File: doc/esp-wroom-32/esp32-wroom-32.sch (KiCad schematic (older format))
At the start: 78 parts, among them Q1 MMFT960, Q2 NDT2955, SW1 Power switch, SW2 Jack plugged, U07 +BATT, U08 +BATT, U1 4066, U1 ESP32-WROOM, U2 MCP23017_SP, U3 MCP1826 5V, U3 MCP23017_SP

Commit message: Documentation.
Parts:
- +1, -1, RF_Module1: symbol esp-wroom-32-rescue:CONN_1-MEGA2560 -> esp32-wroom-32-rescue:CONN_1-MEGA2560-esp-wroom-32-rescue
- .1, .5: symbol esp-wroom-32-rescue:LED-Device -> esp32-wroom-32-rescue:LED-Device-esp-wroom-32-rescue
- .2, ROT_ENC_x1: symbol esp-wroom-32-rescue:SW-MEGA2560 -> esp32-wroom-32-rescue:SW-MEGA2560-esp-wroom-32-rescue
- .3, SW_xx1: symbol esp-wroom-32-rescue:SW_PUSH-MEGA2560 -> esp32-wroom-32-rescue:SW_PUSH-MEGA2560-esp-wroom-32-rescue
- .6, R1, R3, R4, R5, R6, R7, R8, R? (x4): symbol esp-wroom-32-rescue:R-Device -> esp32-wroom-32-rescue:R-Device-esp-wroom-32-rescue
- 101, 102, 103, 104, 105, 3.3V01: symbol esp-wroom-32-rescue:VCC-power -> esp32-wroom-32-rescue:VCC-power-esp-wroom-32-rescue
- C1: symbol esp-wroom-32-rescue:C-Device -> esp32-wroom-32-rescue:C-Device-esp-wroom-32-rescue
- D1: symbol esp-wroom-32-rescue:DIODESCH-MEGA2560 -> esp32-wroom-32-rescue:DIODESCH-MEGA2560-esp-wroom-32-rescue
- GND01: symbol esp-wroom-32-rescue:GND-power -> esp32-wroom-32-rescue:GND-power-esp-wroom-32-rescue
- Pxx1: symbol esp-wroom-32-rescue:POT-MEGA2560 -> esp32-wroom-32-rescue:POT-MEGA2560-esp-wroom-32-rescue
- Q1, Q?: symbol esp-wroom-32-rescue:MOSFET_N-MEGA2560 -> esp32-wroom-32-rescue:MOSFET_N-MEGA2560-esp-wroom-32-rescue
- Q2, Q?: symbol esp-wroom-32-rescue:MOSFET_P-MEGA2560 -> esp32-wroom-32-rescue:MOSFET_P-MEGA2560-esp-wroom-32-rescue
- SW1, SW2: symbol esp-wroom-32-rescue:SPST-MEGA2560 -> esp32-wroom-32-rescue:SPST-MEGA2560-esp-wroom-32-rescue
- U07, U08: symbol esp-wroom-32-rescue:+BATT-power -> esp32-wroom-32-rescue:+BATT-power-esp-wroom-32-rescue
- U1: symbol esp-wroom-32-rescue:4066-MEGA2560 -> esp32-wroom-32-rescue:4066-MEGA2560-esp-wroom-32-rescue
- U1: symbol esp-wroom-32-rescue:ESP32-WROOM-ESP32-footprints-Shem-Lib -> esp32-wroom-32-rescue:ESP32-WROOM-ESP32-footprints-Shem-Lib-esp-wroom-32-rescue
- U2, U3: symbol esp-wroom-32-rescue:MCP23017_SP-Interface_Expansion -> esp32-wroom-32-rescue:MCP23017_SP-Interface_Expansion-esp-wroom-32-rescue
- U3: symbol esp-wroom-32-rescue:7805-MEGA2560 -> esp32-wroom-32-rescue:7805-MEGA2560-esp-wroom-32-rescue
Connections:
- wire segments 261 -> 260
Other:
- note removed: "Pin 9, can be soldered\nwith pin 8 (unused)"

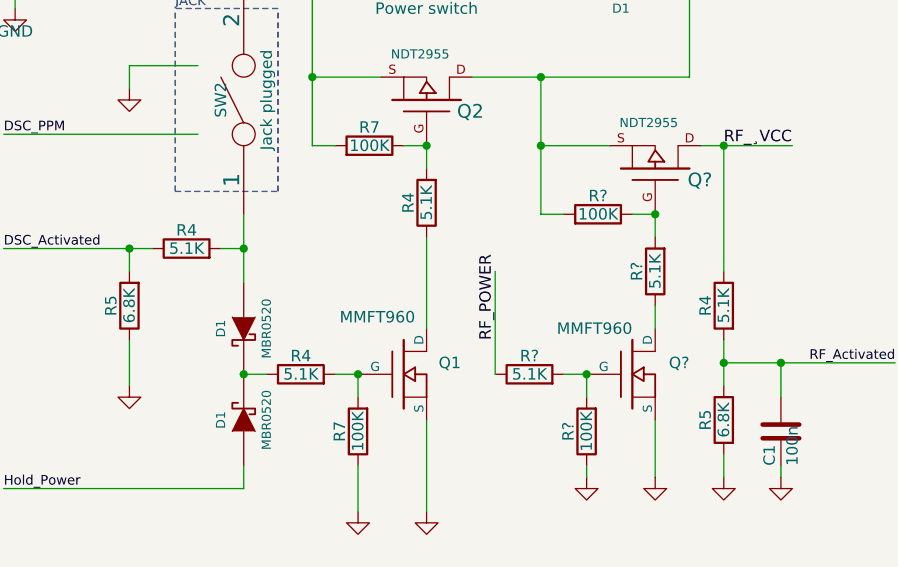
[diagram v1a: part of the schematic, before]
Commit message: Updated schematics & cleanup.
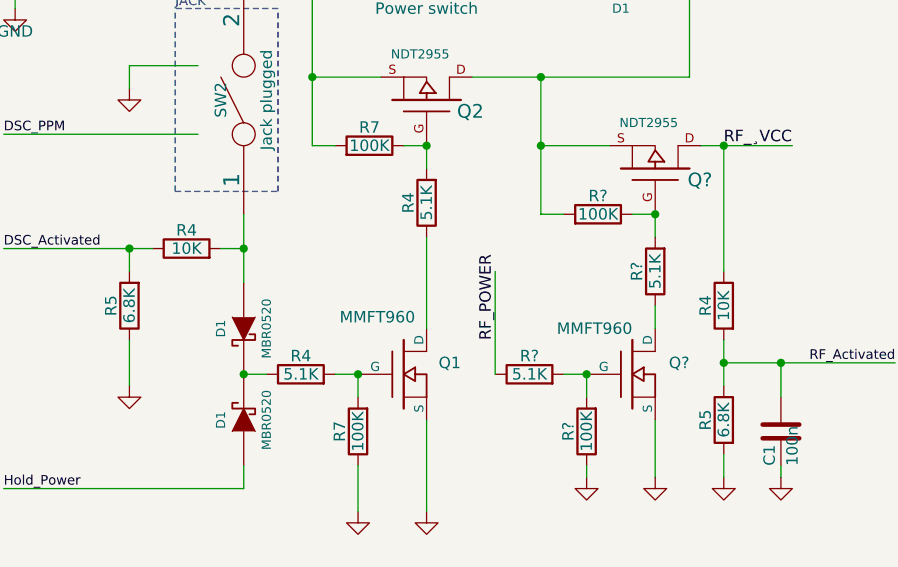
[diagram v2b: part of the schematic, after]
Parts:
- R4: value 5.1K -> 10K
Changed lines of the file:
@@
 P 8000 5000
 F 0 "R4" V 8080 5000 50  0000 C CNN
-F 1 "5.1K" V 8000 5000 50  0000 C CNN
+F 1 "10K" V 8000 5000 50  0000 C CNN
 F 2 "" H 8000 5000 60  0001 C CNN
 F 3 "" H 8000 5000 60  0001 C CNN
@@
 P 10350 5250
 F 0 "R4" V 10430 5250 50  0000 C CNN
-F 1 "5.1K" V 10350 5250 50  0000 C CNN
+F 1 "10K" V 10350 5250 50  0000 C CNN
 F 2 "" H 10350 5250 60  0001 C CNN
 F 3 "" H 10350 5250 60  0001 C CNN
